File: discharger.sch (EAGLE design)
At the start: 109 parts, among them U1 BW6101, U10 BW6101, U11 BW6101, U12 BW6101, U2 BW6101, U3 BW6101, U4 BW6101, U5 BW6101, U6 BW6101, U7 BW6101, U8 BW6101, U9 BW6101

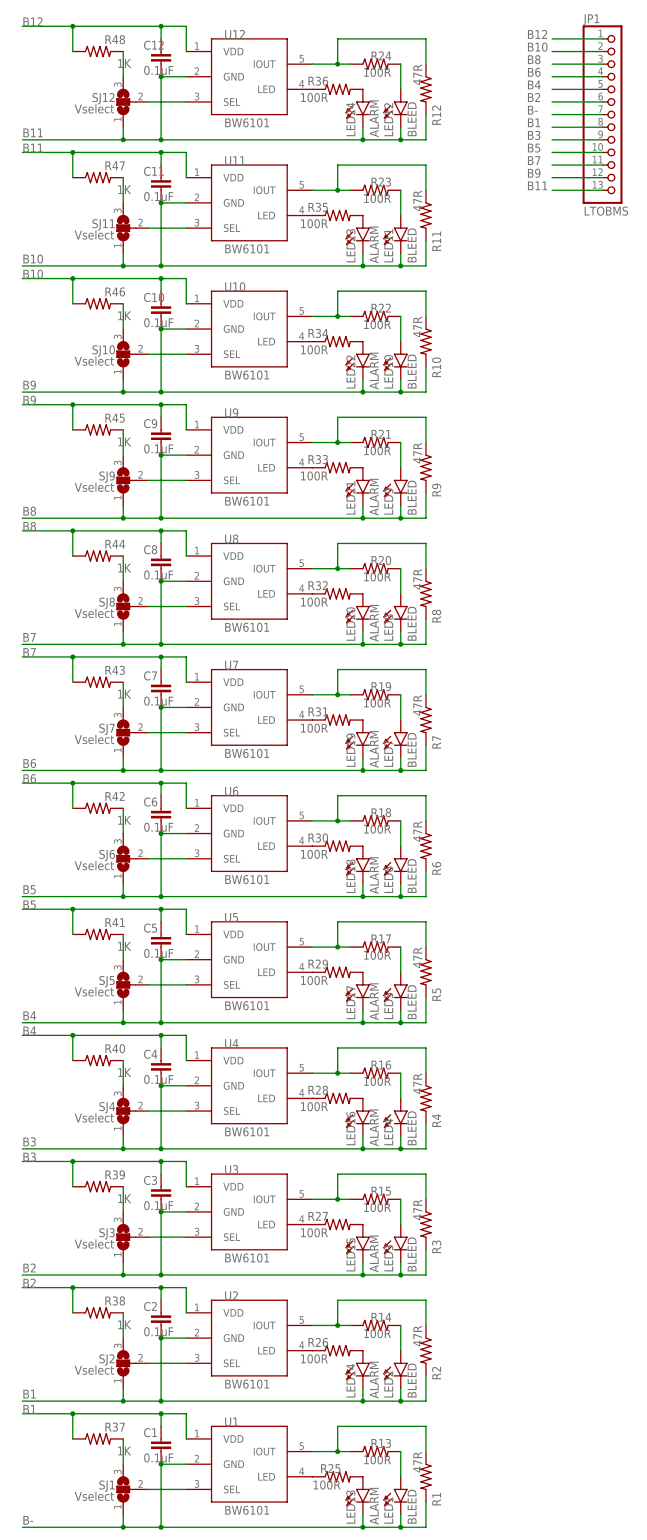
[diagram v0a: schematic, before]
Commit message: move 1k resistor onto SEL side of jumper
more fiddling
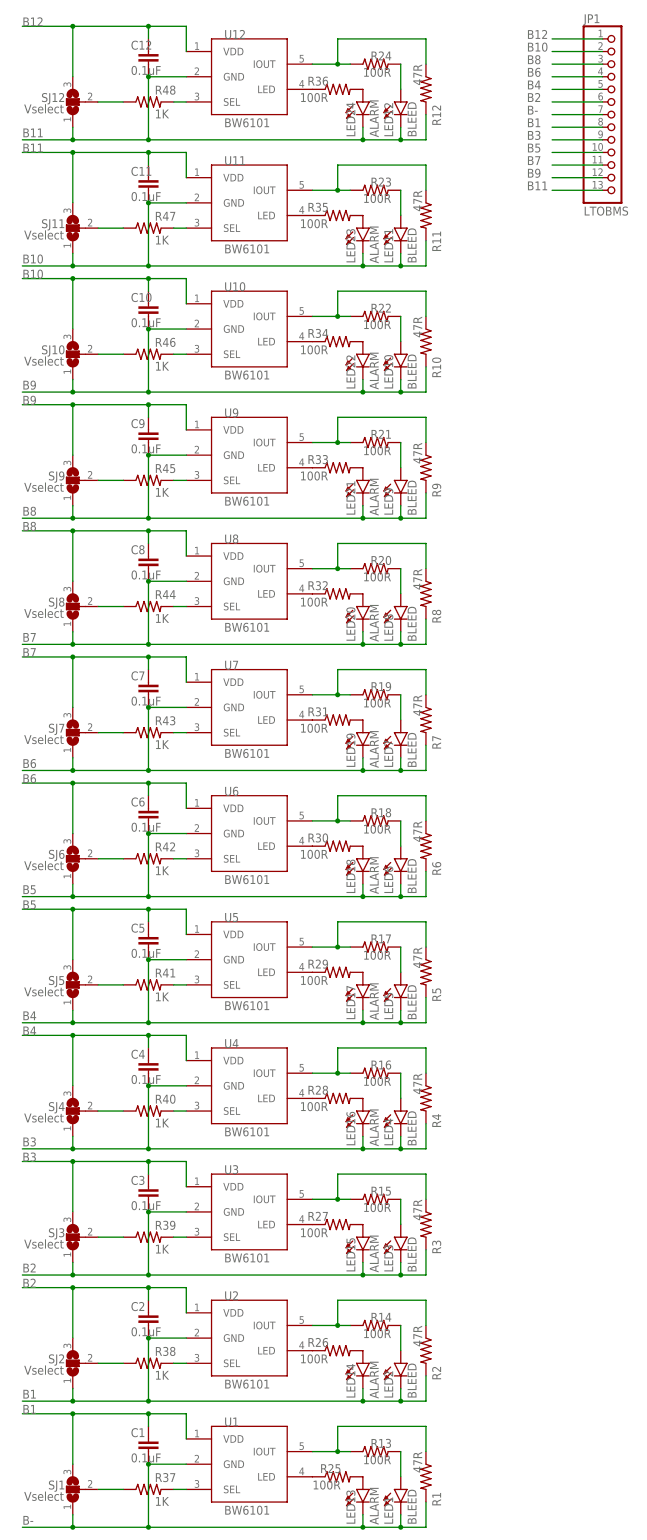
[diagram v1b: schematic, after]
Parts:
- R13, R14, R15, R16, R17, R18, R19, R20, R21, R22, R23, R24, R25, R26, R27, R28, R29, R30, R31, R32, R33, R34, R35, R36: device resistor:R-US_R0805 -> resistor:R-US_R0603
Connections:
- removed net N$72: SJ11.2, U11.SEL
- removed net N$73: R47.2, SJ11.3
- removed net N$82: SJ12.2, U12.SEL
- removed net N$83: R48.2, SJ12.3
- new net N$53: R44.2, U8.SEL
- new net N$54: R43.2, U7.SEL
- new net N$55: R42.2, U6.SEL
- new net N$66: R37.2, U1.SEL
- net B1: now also SJ1.3; no longer R37.1
- net B10: now also SJ10.3; no longer R46.1
- net B11: now also SJ11.3; no longer R47.1
- net B12: now also SJ12.3; no longer R48.1
- net B2: now also SJ2.3; no longer R38.1
- net B3: now also SJ3.3; no longer R39.1
- net B4: now also SJ4.3; no longer R40.1
- net B5: now also SJ5.3; no longer R41.1
- net B6: now also SJ6.3; no longer R42.1
- net B7: now also SJ7.3; no longer R43.1
- net B8: now also SJ8.3; no longer R44.1
- net B9: now also SJ9.3; no longer R45.1
- net N$12: now also R39.1, SJ3.2; no longer SJ1.2, U1.SEL
- net N$13: now also R40.1, SJ4.2; no longer R37.2, SJ1.3
- net N$17: now also R41.1, SJ5.2; no longer SJ8.2, U8.SEL
- net N$18: now also R42.1, SJ6.2; no longer R44.2, SJ8.3
- net N$22: now also R43.1, SJ7.2; no longer SJ2.2, U2.SEL
- net N$23: now also R44.1, SJ8.2; no longer R38.2, SJ2.3
- net N$27: now also R45.1, SJ9.2; no longer SJ4.2, U4.SEL
- net N$28: now also R46.1, SJ10.2; no longer R40.2, SJ4.3
- net N$37: now also R47.1, SJ11.2; no longer SJ5.2, U5.SEL
- net N$38: now also R48.1, SJ12.2; no longer R41.2, SJ5.3
- net N$42: now also R48.2, U12.SEL; no longer SJ9.2, U9.SEL
- net N$43: now also R47.2, U11.SEL; no longer R45.2, SJ9.3
- net N$47: now also R46.2, U10.SEL; no longer SJ6.2, U6.SEL
- net N$48: now also R45.2, U9.SEL; no longer R42.2, SJ6.3
- net N$57: now also R41.2, U5.SEL; no longer SJ7.2, U7.SEL
- net N$58: now also R40.2, U4.SEL; no longer R43.2, SJ7.3
- net N$62: now also R39.2, U3.SEL; no longer SJ10.2, U10.SEL
- net N$63: now also R38.2, U2.SEL; no longer R46.2, SJ10.3
- net N$7: now also R37.1, SJ1.2; no longer SJ3.2, U3.SEL
- net N$8: now also R38.1, SJ2.2; no longer R39.2, SJ3.3
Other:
- moved on the sheet: C1, C10, C11, C12, C2, C3, C4, C5, C6, C7, C8, C9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
